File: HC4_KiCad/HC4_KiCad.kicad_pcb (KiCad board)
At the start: 2 copper layers, 100 x 100 mm, 173 parts, among them IC1 KM62256CLP, IC10 74HC4002, IC11 74HC161, IC12 74HC377, IC13 74HC161, IC14 74HC161, IC15 74HC161, IC16 74HC257, IC17 74HC257, IC18 74HC74, IC19 74HC32, IC2 ROM, IC20 74HC04, IC21 74HC00, IC22 74HC4053, IC23 74HC151, IC24 74HC14, IC3 74HC153, IC4 74HC153, IC5 74HC153, IC6 74HC153, IC7 74HC283, IC8 74HC257, IC9 74HC244, J1 Power, J2 ~{CE}_EXT, J3 Expantion_Connector, SW1 SW_SPDT_312, SW2 Bus_Open, SW3 SW_Push, SW4 SW_Push, SW5 SW_SPDT

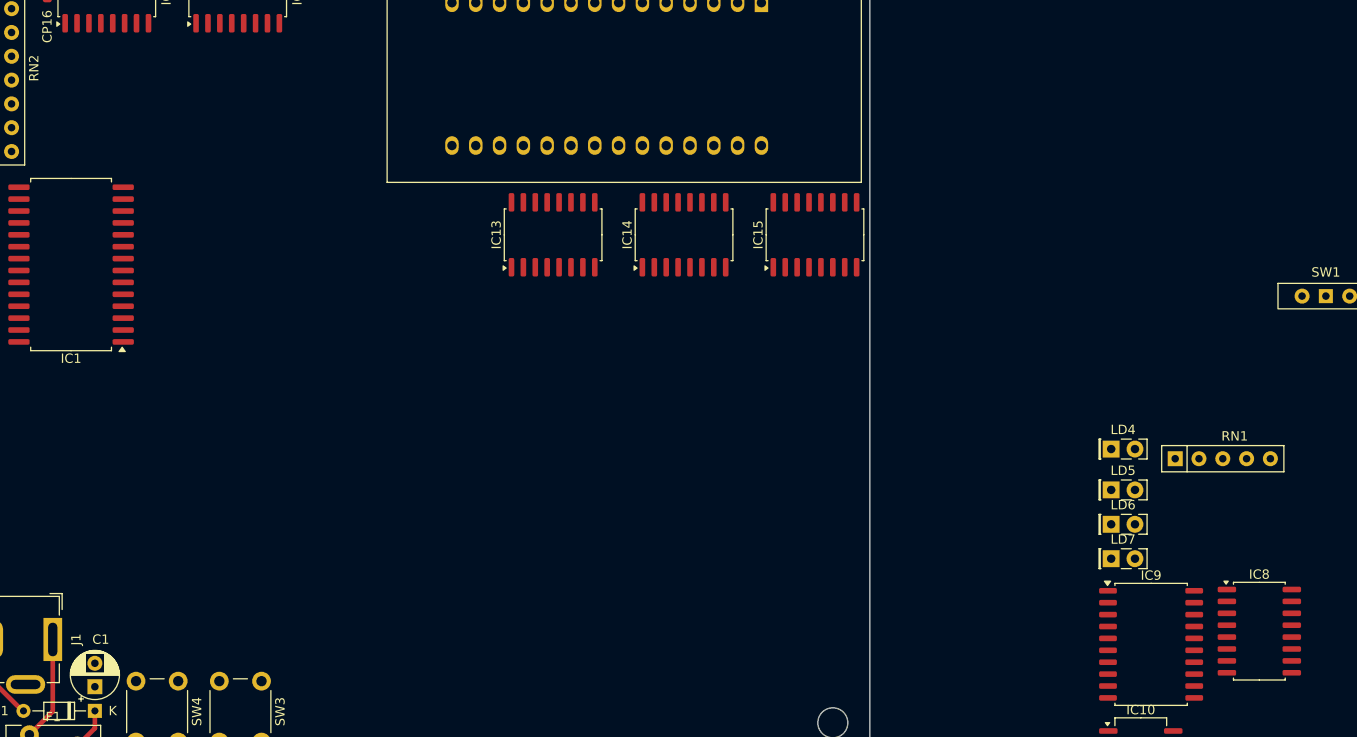
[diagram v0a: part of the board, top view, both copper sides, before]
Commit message: さようなら、爺さん
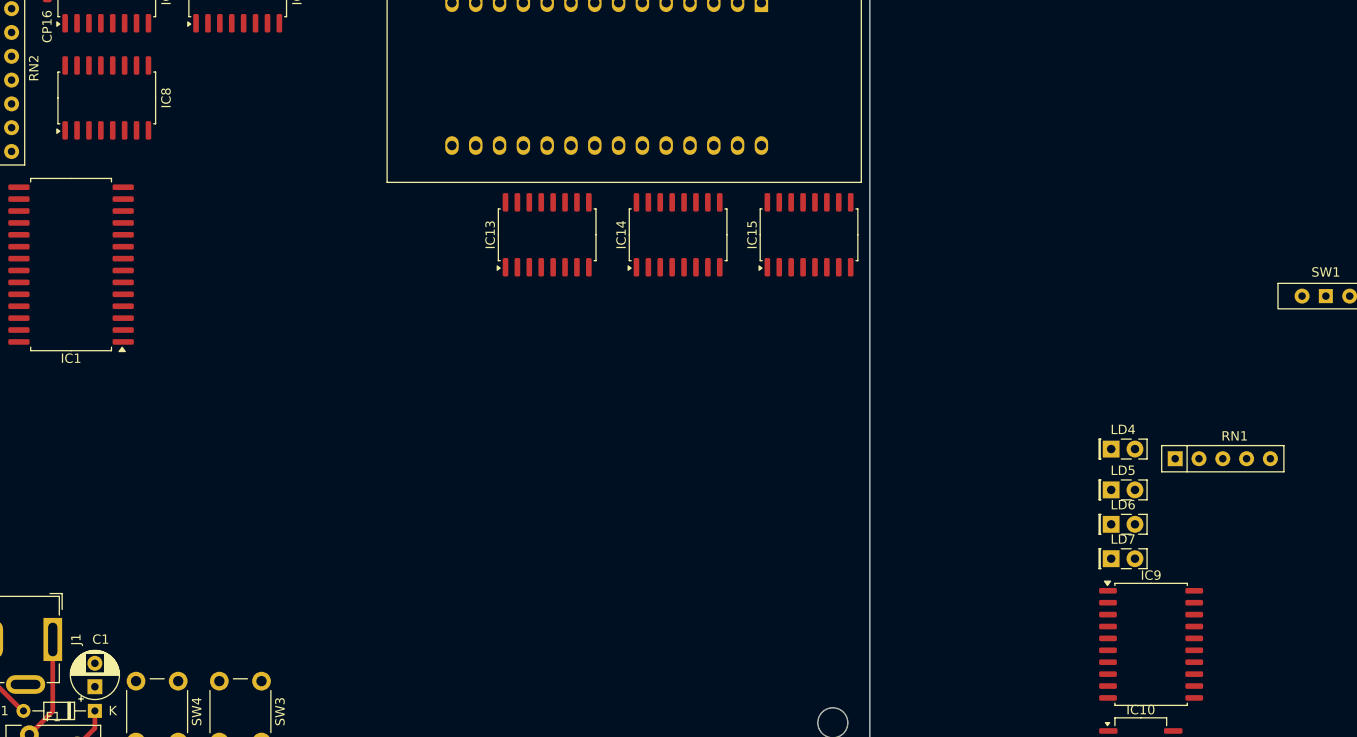
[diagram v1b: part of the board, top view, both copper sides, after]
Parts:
- moved IC8 135.5 mm to (68.6, 79.4), turned to 90 degrees
- moved IC14 0.64 mm to (129.5, 94.0)
- moved IC15 0.64 mm to (143.5, 94.0)
- moved IC13 0.64 mm to (115.6, 94.0)
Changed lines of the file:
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@@
 	(footprint "Package_SO:SO-16_5.3x10.2mm_P1.27mm"
 		(layer "F.Cu")
-		(at 130.175 93.98 90)
+		(at 129.54 93.98 90)
 		(descr "SO, 16 Pin (https://www.ti.com/lit/ml/msop002a/msop002a.pdf), generated with kicad-footprint-generator ipc_gullwing_generator.py")
 		(tags "SO SO")
@@
 	(footprint "Package_SO:SO-16_5.3x10.2mm_P1.27mm"
 		(layer "F.Cu")
-		(at 116.205 93.98 90)
+		(at 115.57 93.98 90)
 		(descr "SO, 16 Pin (https://www.ti.com/lit/ml/msop002a/msop002a.pdf), generated with kicad-footprint-generator ipc_gullwing_generator.py")
 		(tags "SO SO")
@@
 		(tags "LED")
 		(property "Reference" "LD4"
-			(at 1.27 -2.06 360)
+			(at 1.27 -2.06 0)
 			(layer "F.SilkS")
 			(effects
@@
 		)
 		(property "Value" "LED"
-			(at 1.27 2.06 360)
+			(at 1.27 2.06 0)
 			(layer "F.Fab")
 			(effects
@@
 		)
 		(property "Footprint" "LED_THT:LED_Rectangular_W5.0mm_H2.0mm"
-			(at 0 0 360)
+			(at 0 0 0)
 			(layer "F.Fab")
 			(hide yes)
@@
 		)
 		(property "Datasheet" ""
-			(at 0 0 360)
+			(at 0 0 0)
 			(layer "F.Fab")
 			(hide yes)
@@
 		)
 		(property "Description" "Light emitting diode"
-			(at 0 0 360)
+			(at 0 0 0)
 			(layer "F.Fab")
 			(hide yes)
@@
 		)
 		(fp_text user "${REFERENCE}"
-			(at 1.27 0 360)
+			(at 1.27 0 0)
 			(layer "F.Fab")
 			(effects
@@
 		(tags "Diode DO-34_SOD68 series Axial Horizontal pin pitch 7.62mm  length 3.04mm diameter 1.6mm")
 		(property "Reference" "D1"
-			(at 10.16 0 360)
+			(at 10.16 0 0)
 			(layer "F.SilkS")
 			(effects
@@
 		)
 		(property "Value" "5.6V"
-			(at 3.81 1.92 360)
+			(at 3.81 1.92 0)
 			(layer "F.Fab")
 			(effects
@@
 		)
 		(fp_text user "K"
-			(at -1.905 0 360)
+			(at -1.905 0 0)
 			(layer "F.SilkS")
 			(effects
@@
 		)
 		(fp_text user "K"
-			(at 0 -1.75 360)
+			(at 0 -1.75 0)
 			(layer "F.Fab")
 			(effects
@@
 		)
 		(fp_text user "${REFERENCE}"
-			(at 4.038 0 360)
+			(at 4.038 0 0)
 			(layer "F.Fab")
 			(effects
@@
 		(tags "LED")
 		(property "Reference" "LD32"
-			(at -3.81 0 360)
+			(at -3.81 0 0)
 			(layer "F.SilkS")
 			(effects
@@
 	(footprint "Package_SO:SO-16_5.3x10.2mm_P1.27mm"
 		(layer "F.Cu")
-		(at 191.56 136.27)
+		(at 68.58 79.375 90)
 		(descr "SO, 16 Pin (https://www.ti.com/lit/ml/msop002a/msop002a.pdf), generated with kicad-footprint-generator ipc_gullwing_generator.py")
 		(tags "SO SO")
 		(property "Reference" "IC8"
-			(at 0 -6.05 0)
+			(at 0 6.35 90)
 			(layer "F.SilkS")
 			(effects
@@
 		)
 		(property "Value" "74HC257"
-			(at 0 6.05 0)
+			(at 0 6.05 90)
 			(layer "F.Fab")
 			(effects
@@
 		)
 		(property "Footprint" "Package_SO:SO-16_5.3x10.2mm_P1.27mm"
-			(at 0 0 0)
+			(at 0 0 90)
 			(layer "F.Fab")
 			(hide yes)
@@
 		)
 		(property "Datasheet" "http://www.ti.com/lit/gpn/sn74LS257"
-			(at 0 0 0)
+			(at 0 0 90)
 			(layer "F.Fab")
 			(hide yes)
@@
 		)
 		(property "Description" "Quad 2 to 1 Multiplexer"
-			(at 0 0 0)
+			(at 0 0 90)
 			(layer "F.Fab")
 			(hide yes)
@@
 		(attr smd)
 		(fp_line
-			(start -2.76 -5.21)
-			(end -2.76 -5.005)
+			(start 2.76 -5.21)
+			(end 2.76 -5.005)
 			(stroke
 				(width 0.12)
@@
 		)
 		(fp_line
-			(start -2.76 5.21)
-			(end -2.76 5.005)
+			(start 0 -5.21)
+			(end 2.76 -5.21)
 			(stroke
 				(width 0.12)
@@
 		)
 		(fp_line
-			(start 0 -5.21)
-			(end 2.76 -5.21)
+			(start -2.76 -5.21)
+			(end -2.76 -5.005)
 			(stroke
 				(width 0.12)
@@
 		)
 		(fp_line
-			(start 0 5.21)
-			(end -2.76 5.21)
+			(start 2.76 5.21)
+			(end 2.76 5.005)
 			(stroke
 				(width 0.12)
@@
 		)
 		(fp_line
-			(start 2.76 -5.21)
-			(end 2.76 -5.005)
+			(start 0 5.21)
+			(end -2.76 5.21)
 			(stroke
 				(width 0.12)
@@
 		)
 		(fp_line
-			(start 2.76 5.21)
-			(end 2.76 5.005)
+			(start -2.76 5.21)
+			(end -2.76 5.005)
 			(stroke
 				(width 0.12)
@@
 		)
 		(fp_line
-			(start -4.7 -5.35)
-			(end -4.7 5.35)
+			(start 4.7 -5.35)
+			(end -4.7 -5.35)
 			(stroke
 				(width 0.05)
@@
 		)
 		(fp_line
-			(start -4.7 5.35)
-			(end 4.7 5.35)
+			(start -4.7 -5.35)
+			(end -4.7 5.35)
 			(stroke
 				(width 0.05)
@@
 		)
 		(fp_line
-			(start 4.7 -5.35)
-			(end -4.7 -5.35)
+			(start 4.7 5.35)
+			(end 4.7 -5.35)
 			(stroke
 				(width 0.05)
@@
 		)
 		(fp_line
-			(start 4.7 5.35)
-			(end 4.7 -5.35)
+			(start -4.7 5.35)
+			(end 4.7 5.35)
 			(stroke
 				(width 0.05)
@@
 		)
 		(fp_line
-			(start -2.65 -4.1)
-			(end -1.65 -5.1)
+			(start 2.65 -5.1)
+			(end 2.65 5.1)
 			(stroke
 				(width 0.1)
@@
 		)
 		(fp_line
-			(start -2.65 5.1)
-			(end -2.65 -4.1)
+			(start -1.65 -5.1)
+			(end 2.65 -5.1)
 			(stroke
 				(width 0.1)
@@
 		)
 		(fp_line
-			(start -1.65 -5.1)
-			(end 2.65 -5.1)
+			(start -2.65 -4.1)
+			(end -1.65 -5.1)
 			(stroke
 				(width 0.1)
@@
 		)
 		(fp_line
-			(start 2.65 -5.1)
-			(end 2.65 5.1)
+			(start 2.65 5.1)
+			(end -2.65 5.1)
 			(stroke
 				(width 0.1)
@@
 		)
 		(fp_line
-			(start 2.65 5.1)
-			(end -2.65 5.1)
+			(start -2.65 5.1)
+			(end -2.65 -4.1)
 			(stroke
 				(width 0.1)
@@
 		)
 		(fp_text user "${REFERENCE}"
-			(at 0 0 0)
+			(at 0 0 90)
 			(layer "F.Fab")
 			(effects
@@
 		)
 		(pad "1" smd roundrect
-			(at -3.4625 -4.445)
+			(at -3.4625 -4.445 90)
 			(size 1.975 0.6)
 			(layers "F.Cu" "F.Paste" "F.Mask")
@@
 		)
 		(pad "2" smd roundrect
-			(at -3.4625 -3.175)
+			(at -3.4625 -3.175 90)
 			(size 1.975 0.6)
 			(layers "F.Cu" "F.Paste" "F.Mask")
@@
 		)
 		(pad "3" smd roundrect
-			(at -3.4625 -1.905)
+			(at -3.4625 -1.905 90)
 			(size 1.975 0.6)
 			(layers "F.Cu" "F.Paste" "F.Mask")
@@
 		)
 		(pad "4" smd roundrect
-			(at -3.4625 -0.635)
+			(at -3.4625 -0.635 90)
 			(size 1.975 0.6)
 			(layers "F.Cu" "F.Paste" "F.Mask")
@@
 		)
 		(pad "5" smd roundrect
-			(at -3.4625 0.635)
+			(at -3.4625 0.635 90)
 			(size 1.975 0.6)
 			(layers "F.Cu" "F.Paste" "F.Mask")
@@
 		)
 		(pad "6" smd roundrect
-			(at -3.4625 1.905)
+			(at -3.4625 1.905 90)
 			(size 1.975 0.6)
 			(layers "F.Cu" "F.Paste" "F.Mask")
@@
 		)
 		(pad "7" smd roundrect
-			(at -3.4625 3.175)
+			(at -3.4625 3.175 90)
 			(size 1.975 0.6)
 			(layers "F.Cu" "F.Paste" "F.Mask")
@@
 		)
 		(pad "8" smd roundrect
-			(at -3.4625 4.445)
+			(at -3.4625 4.445 90)
 			(size 1.975 0.6)
 			(layers "F.Cu" "F.Paste" "F.Mask")
@@
 		)
 		(pad "9" smd roundrect
-			(at 3.4625 4.445)
+			(at 3.4625 4.445 90)
 			(size 1.975 0.6)
 			(layers "F.Cu" "F.Paste" "F.Mask")
@@
 		)
 		(pad "10" smd roundrect
-			(at 3.4625 3.175)
+			(at 3.4625 3.175 90)
 			(size 1.975 0.6)
 			(layers "F.Cu" "F.Paste" "F.Mask")
@@
 		)
 		(pad "11" smd roundrect
-			(at 3.4625 1.905)
+			(at 3.4625 1.905 90)
 			(size 1.975 0.6)
 			(layers "F.Cu" "F.Paste" "F.Mask")
@@
 		)
 		(pad "12" smd roundrect
-			(at 3.4625 0.635)
+			(at 3.4625 0.635 90)
 			(size 1.975 0.6)
 			(layers "F.Cu" "F.Paste" "F.Mask")
@@
 		)
 		(pad "13" smd roundrect
-			(at 3.4625 -0.635)
+			(at 3.4625 -0.635 90)
 			(size 1.975 0.6)
 			(layers "F.Cu" "F.Paste" "F.Mask")
@@
 		)
 		(pad "14" smd roundrect
-			(at 3.4625 -1.905)
+			(at 3.4625 -1.905 90)
 			(size 1.975 0.6)
 			(layers "F.Cu" "F.Paste" "F.Mask")
@@
 		)
 		(pad "15" smd roundrect
-			(at 3.4625 -3.175)
+			(at 3.4625 -3.175 90)
 			(size 1.975 0.6)
 			(layers "F.Cu" "F.Paste" "F.Mask")
@@
 		)
 		(pad "16" smd roundrect
-			(at 3.4625 -4.445)
+			(at 3.4625 -4.445 90)
 			(size 1.975 0.6)
 			(layers "F.Cu" "F.Paste" "F.Mask")
@@
 		(tags "ptc resettable fuse polyfuse THT")
 		(property "Reference" "F1"
-			(at 2.54 -1.905 360)
+			(at 2.54 -1.905 0)
 			(layer "F.SilkS")
 			(effects
@@
 		)
 		(property "Value" "Polyfuse"
-			(at 2.55 3.1 360)
+			(at 2.55 3.1 0)
 			(layer "F.Fab")
 			(effects
@@
 		)
 		(fp_text user "${REFERENCE}"
-			(at 2.55 0.6 360)
+			(at 2.55 0.6 0)
 			(layer "F.Fab")
 			(effects
@@
 	(footprint "Package_SO:SO-16_5.3x10.2mm_P1.27mm"
 		(layer "F.Cu")
-		(at 144.145 93.98 90)
+		(at 143.51 93.98 90)
 		(descr "SO, 16 Pin (https://www.ti.com/lit/ml/msop002a/msop002a.pdf), generated with kicad-footprint-generator ipc_gullwing_generator.py")
 		(tags "SO SO")
@@
 		(tags "THT DIP DIL ZIF 15.24mm 600mil Socket")
 		(property "Reference" "IC2"
-			(at -5.08 -10.16 360)
+			(at -5.08 -10.16 0)
 			(layer "F.SilkS")
 			(effects
